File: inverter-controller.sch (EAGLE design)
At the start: 190 parts, among them IC1 STM32F334C8T6, IC2 SY7152ABC, IC3 LMV358MMX, IC4 LMV358MMX, IC5 SY7152ABC, J1 621006245821, J2 61300211121, J3 MCV3, J4 MCV3, J5 MCV3, K1 FINDER_34.51.7.024.0010FINDER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, K2 FINDER_34.51.7.024.0010FINDER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, K3 FINDER_34.51.7.024.0010FINDER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, U1 DIODES_AP3015KTR-G1DIODES_AP3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, X1 0289-9066**15EDGVC-3.81-02P-14, X2 0289-9066**15EDGVC-3.81-02P-14, X3 0289-9066**15EDGVC-3.81-02P-14, X4 0289-9066**15EDGVC-3.81-02P-14, X5 1365-10, X6 1365-16, X7 1365-10, X8 1365-10, Y1 NX2016SA-32M

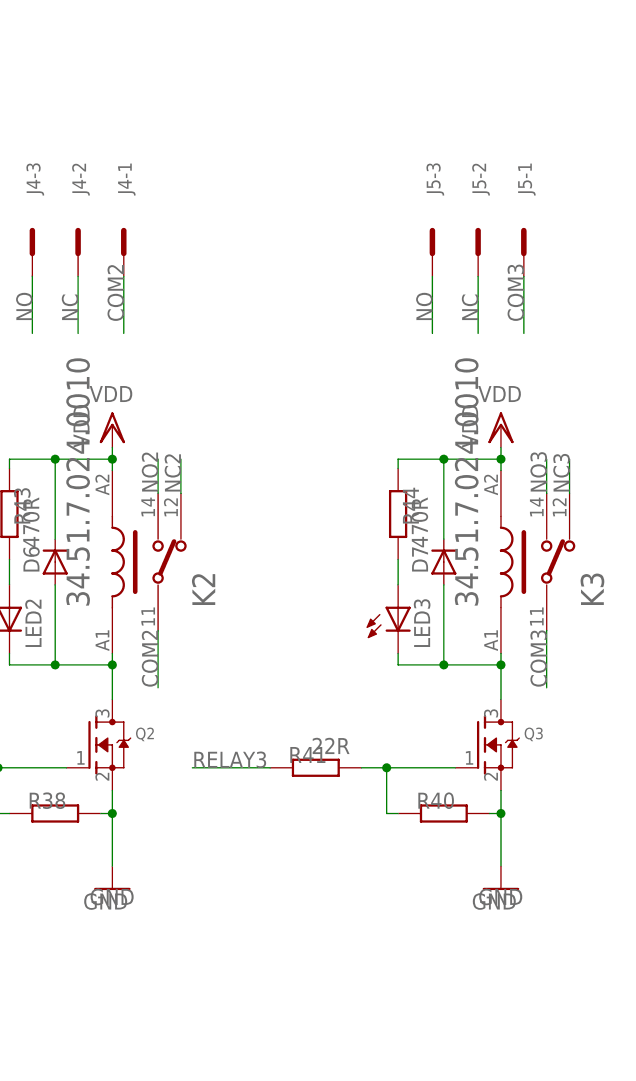
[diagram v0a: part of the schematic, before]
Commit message: Mekanik kistaslar belirlendi.
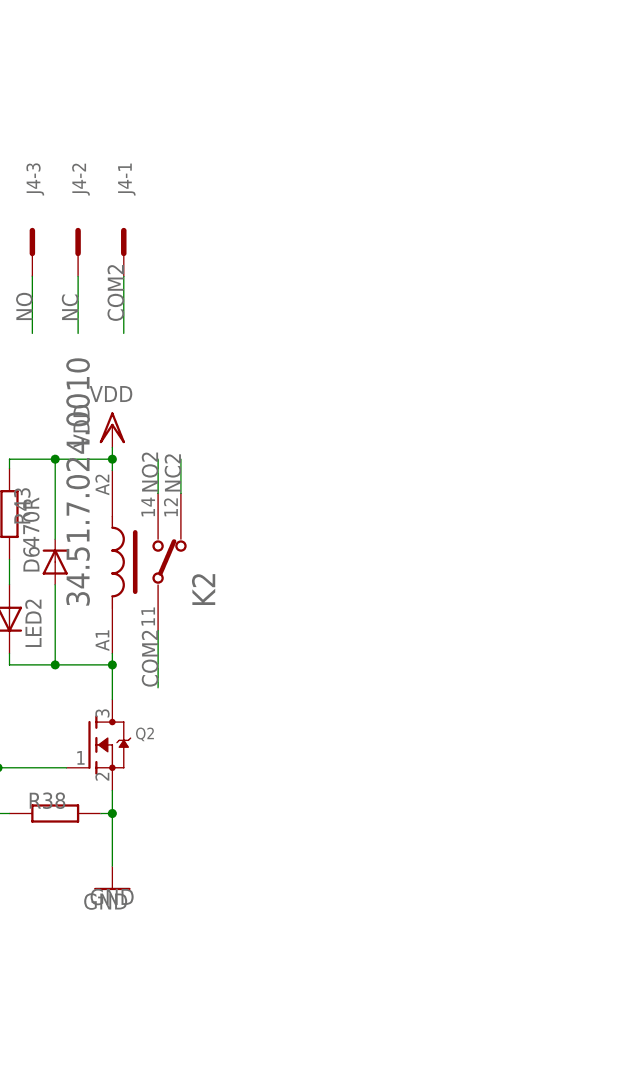
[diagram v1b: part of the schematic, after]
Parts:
- removed D7: (no value), diode:DIODE-SOD80C
- removed J5: MCV3, con-phoenix-381:MCV3
- removed K3: FINDER_34.51.7.024.0010FINDER_34.51.7.024.0010_0_0, Finder - 34.51.7.024.0010:FINDER_34.51.7.024.0010FINDER_34.51.7.024.0010_0_0
- removed LED3: (no value), adafruit:LEDCHIPLED_0805
- removed Q3: (no value), adafruit:MOSFET-NREFLOW
- removed R40: (no value), rcl:R-EU_R0603
- removed R41: 22R, rcl:R-EU_R0603
- removed R44: 470R, rcl:R-EU_R0603
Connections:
- removed net COM3: J5-1.SK, K3.11
- removed net N$28: Q3.G, R40.2, R41.1
- removed net N$31: D7.A, K3.A1, LED3.C, Q3.D
- removed net N$33: LED3.A, R44.1
- removed net NC3: K3.12
- removed net NO3: K3.14
- net GND: no longer Q3.S, R40.1
- net NC: no longer J5-2.SK
- net NO: no longer J5-3.SK
- net RELAY3: no longer R41.2
- net VDD: no longer D7.C, K3.A2, R44.2
